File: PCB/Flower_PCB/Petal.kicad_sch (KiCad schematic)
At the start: 102 parts, among them J1 Conn_01x02_Pin, J2 Conn_01x02_Pin, J3 Conn_01x02_Pin, J4 Conn_01x02_Pin, J5 Conn_01x02_Pin, J6 Conn_01x02_Pin

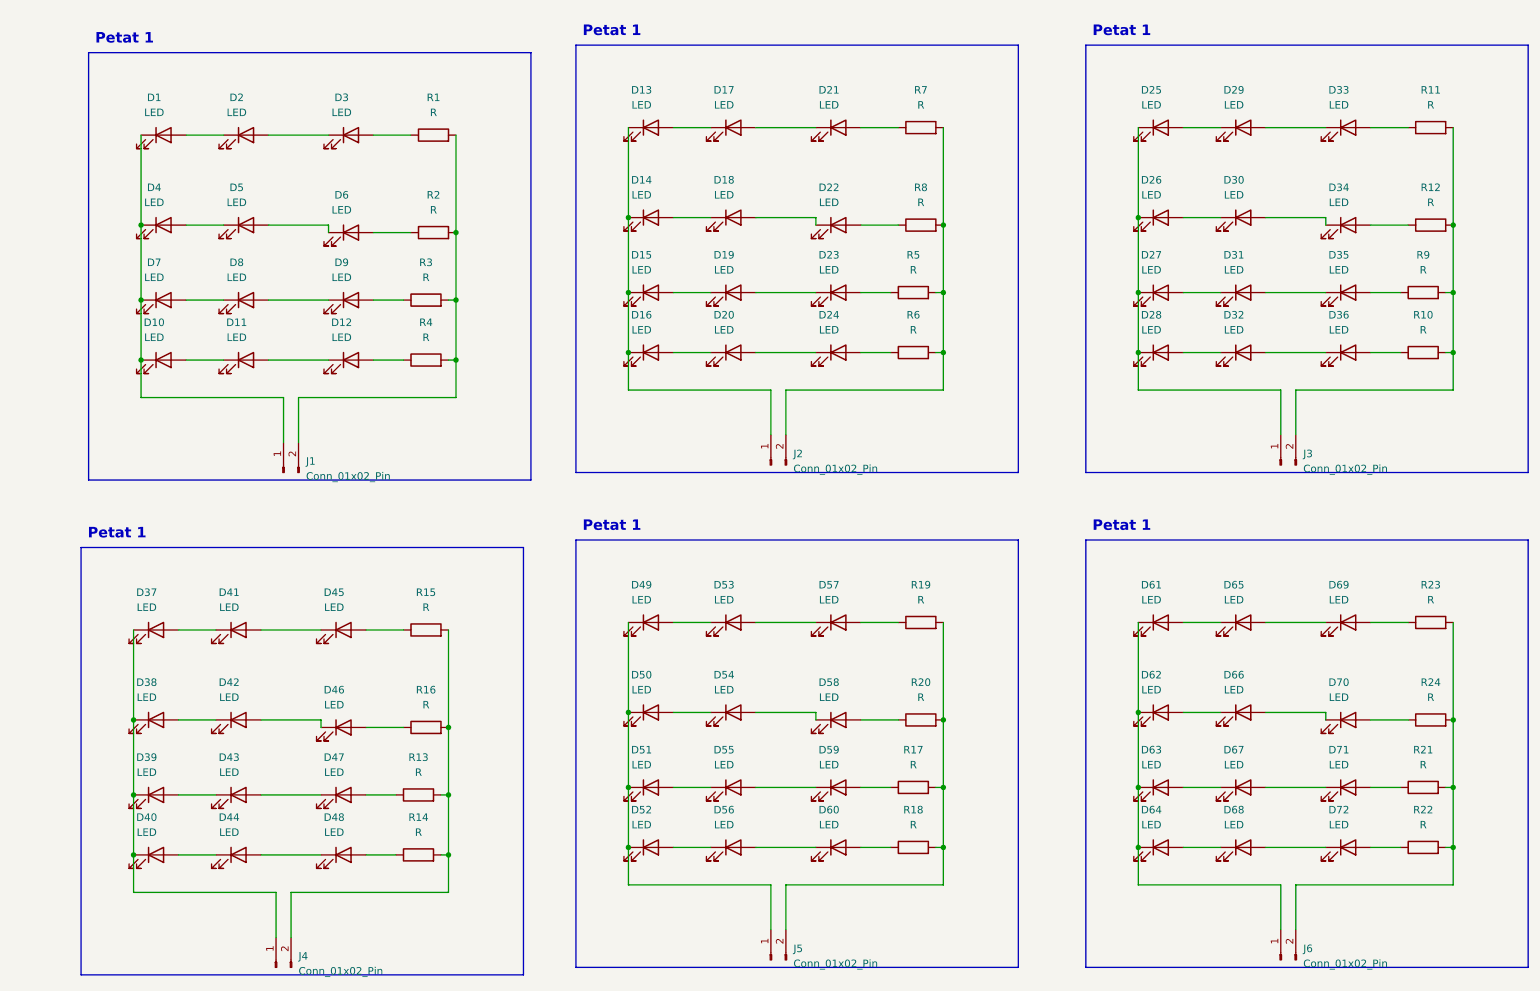
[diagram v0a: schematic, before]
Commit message: the petal designe has been updated
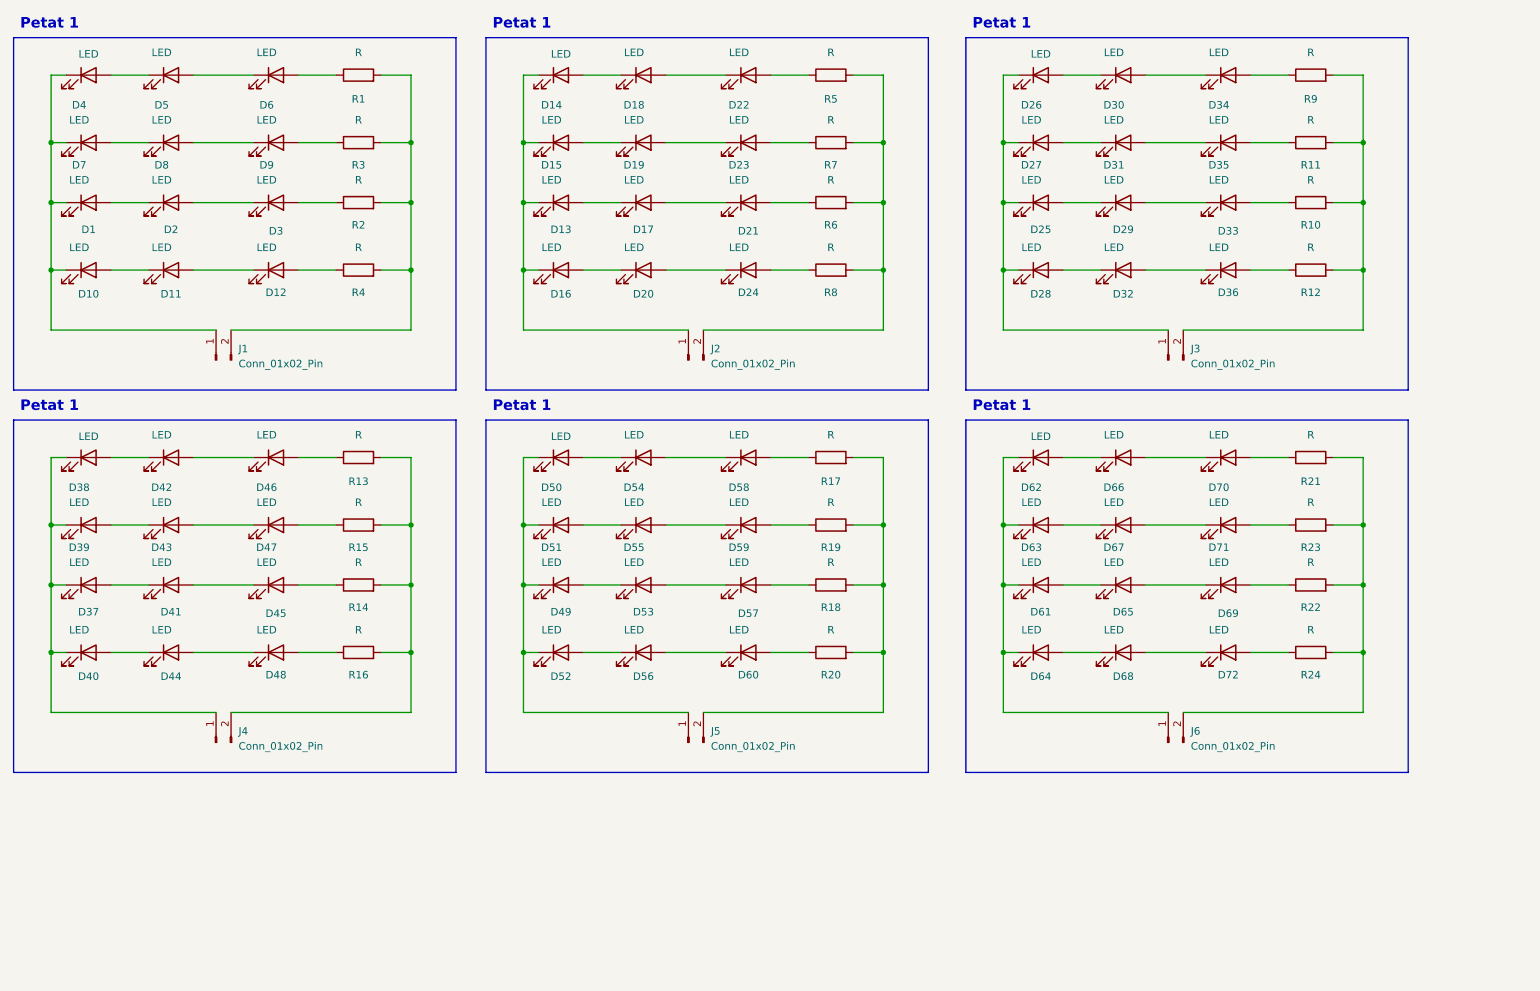
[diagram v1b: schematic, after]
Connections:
- net at R7.1: now also D23.2 (A); no longer D21.2 (A)
- net at R14.1: now also D46.2 (A); no longer D48.2 (A)
- net at R16.1: now also D48.2 (A); no longer D46.2 (A)
- net at R18.1: now also D58.2 (A); no longer D60.2 (A)
- net at D47.2 (A): now also R15.1; no longer R13.1
- net at R10.1: now also D34.2 (A); no longer D36.2 (A)
- net at D33.2 (A): now also R9.1; no longer R11.1
- net at R21.1: now also D69.2 (A); no longer D71.2 (A)
- net at D72.2 (A): now also R24.1; no longer R22.1
- net at D59.2 (A): now also R19.1; no longer R17.1
- net at D35.2 (A): now also R11.1; no longer R9.1
- net at D45.2 (A): now also R13.1; no longer R15.1
- net at D24.2 (A): now also R8.1; no longer R6.1
- net at R5.1: now also D21.2 (A); no longer D23.2 (A)
- net at R12.1: now also D36.2 (A); no longer D34.2 (A)
- net at R23.1: now also D71.2 (A); no longer D69.2 (A)
- net at D22.2 (A): now also R6.1; no longer R8.1
- net at R20.1: now also D60.2 (A); no longer D58.2 (A)
- net at D57.2 (A): now also R17.1; no longer R19.1
- net at D70.2 (A): now also R22.1; no longer R24.1
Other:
- moved on the sheet: D1, D2, D3, D4, D5, D6, D7, D8, D9, J1, R1, R2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
